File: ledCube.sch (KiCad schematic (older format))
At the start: 13 parts, among them P1 CONN_01X03, P2 CONN_01X02, P3 CONN_01X02, P4 CONN_01X02, P5 CONN_01X02, U1 AL8805W5

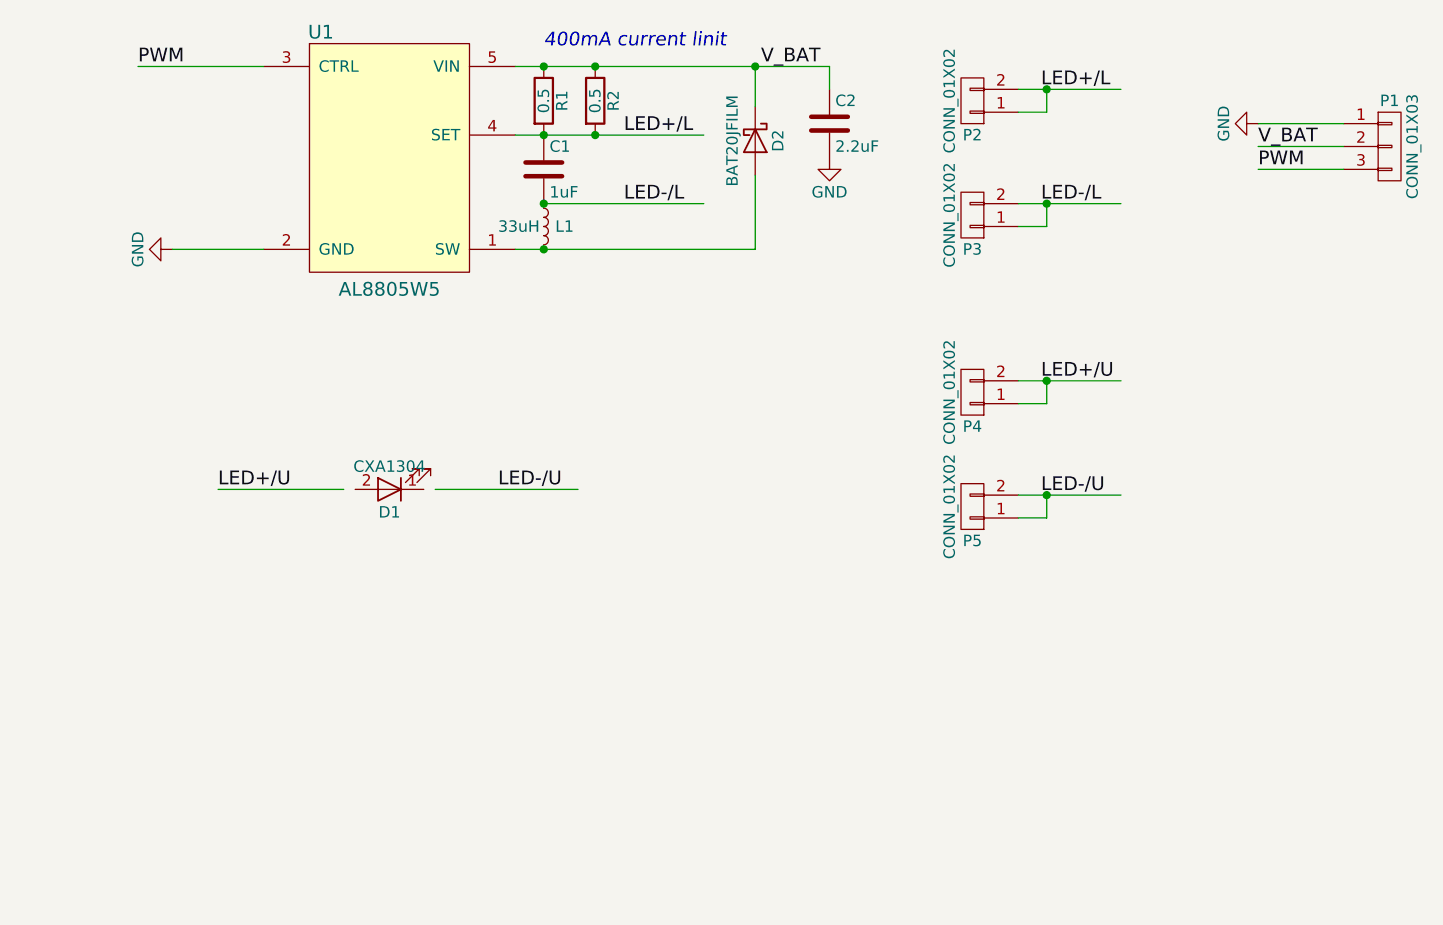
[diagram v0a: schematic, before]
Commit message: Generate BOM & Gerber
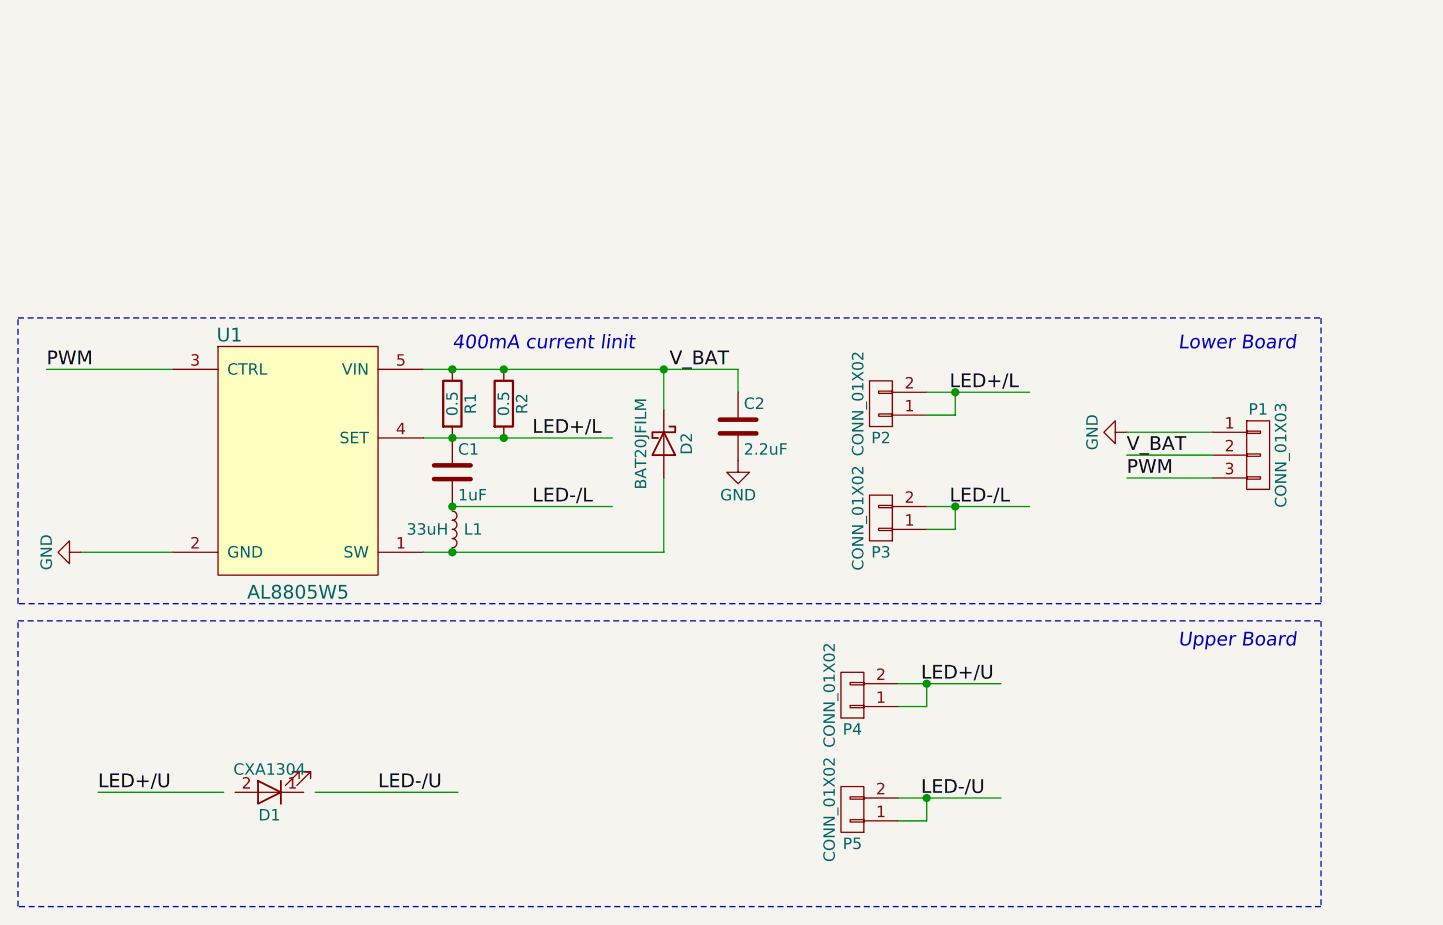
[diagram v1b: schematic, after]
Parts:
- R1, R2: Part # (none) -> 311-0.5LWCT-ND; Vender (none) -> DigiKey
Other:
- note added: "Lower Board"
- note added: "Upper Board"
- moved on the sheet: C1, C2, D1, D2, L1, P1, P2, P3, P4, P5, R1, R2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
